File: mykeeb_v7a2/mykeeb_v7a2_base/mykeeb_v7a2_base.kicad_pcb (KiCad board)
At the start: 2 copper layers, 162.4 x 130 mm, 38 parts

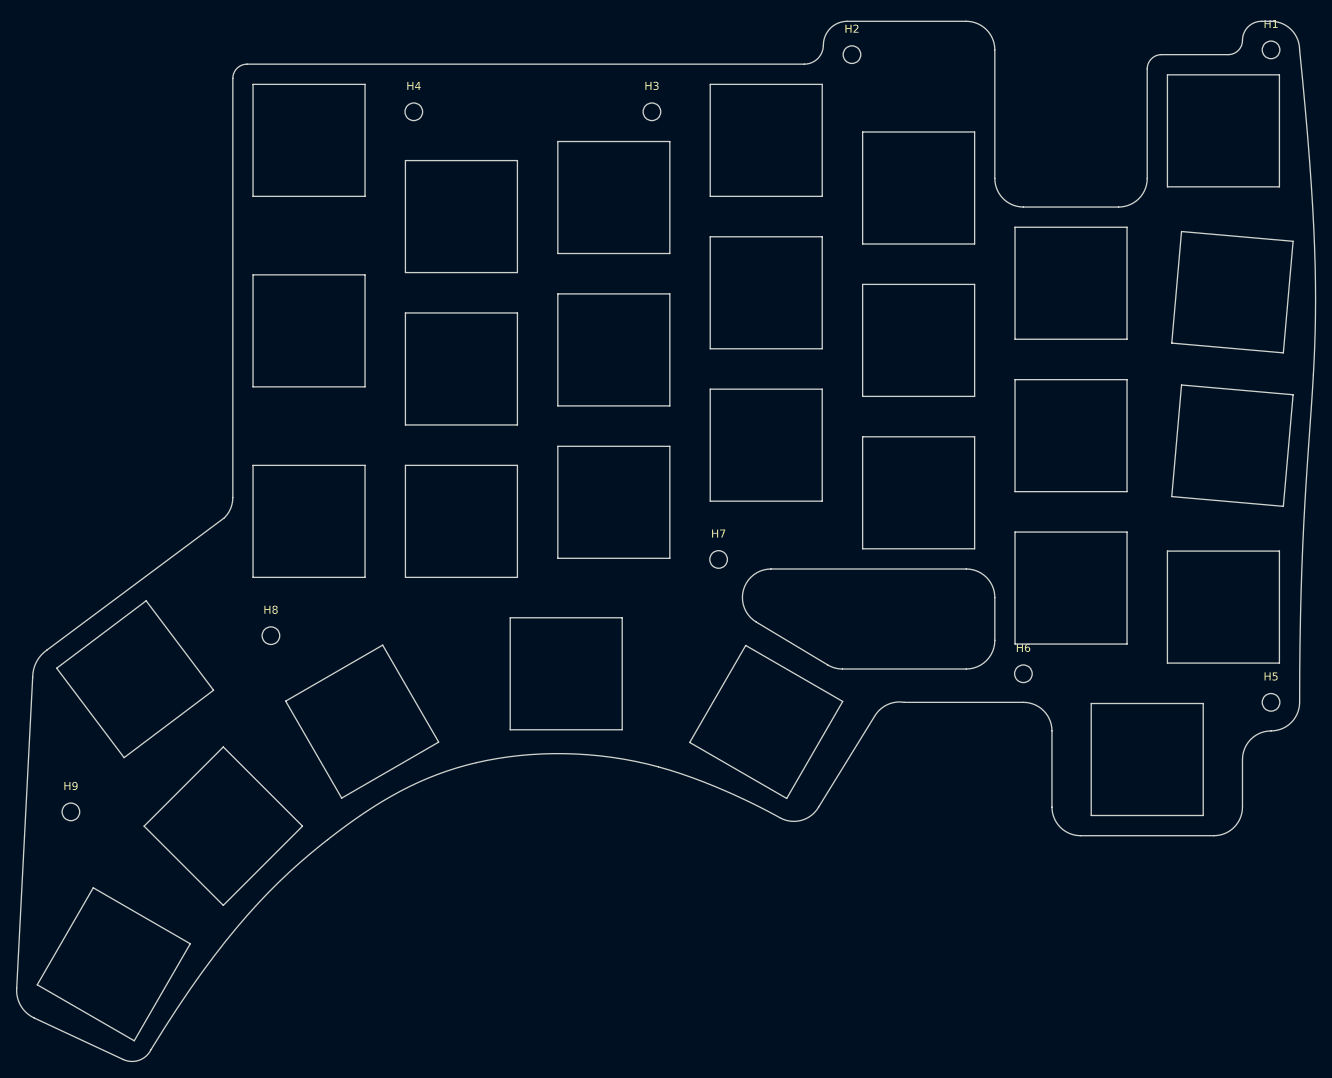
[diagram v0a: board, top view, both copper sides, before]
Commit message: add gerber files for v7a2
Signed-off-by: Maximilian Huber <gh@maxhbr.de>
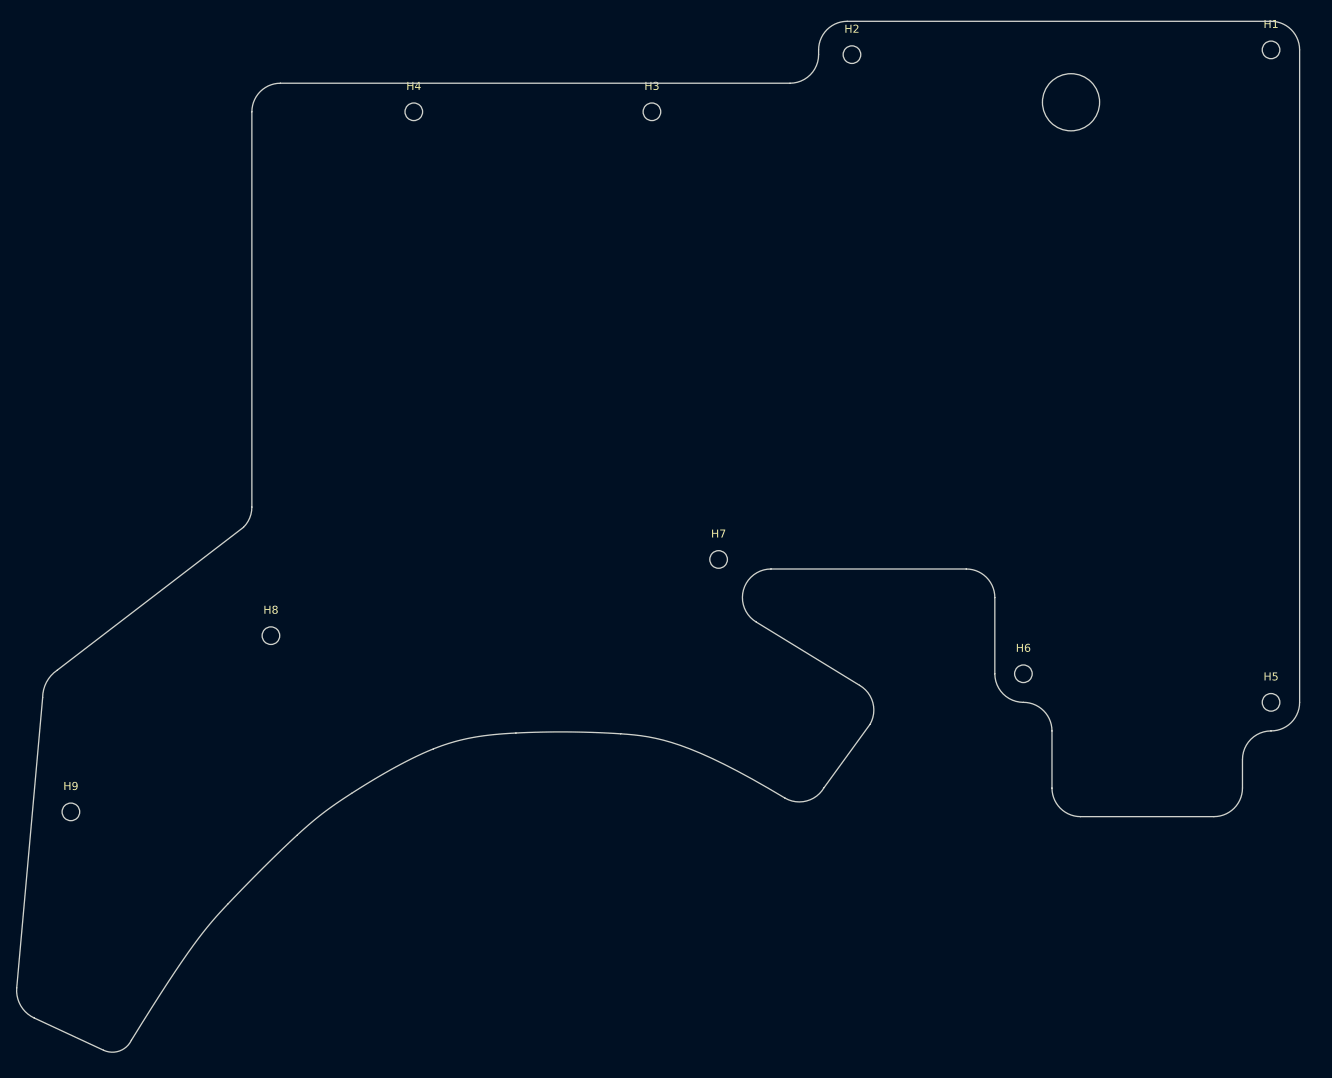
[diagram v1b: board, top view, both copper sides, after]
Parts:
- removed S0, S10, S11, S12, S13, S14, S15, S2, S20, S21, S22, S23, S24, S25, S3, S30, S31, S32, S33, S34, S35, S4, S40, S42, S43, S44, S5, locked (x2): SW, pretty:SW_Hole
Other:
- board size 162.4 x 130 mm -> 160.4 x 128.9 mm
